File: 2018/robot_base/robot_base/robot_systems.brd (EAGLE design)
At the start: 102.8 x 91.4 mm, 92 parts, among them IC1 DRV8840PWP, IC1_C1 0.01uF, IC1_C2 0.1uF, IC1_C3 0.1uF, IC1_C4 0.1uF, IC1_C5 100uF, IC1_C6 470nF, IC1_R1 ???, IC1_R2 ???, IC1_R3 10k, IC1_R4 100m, IC1_R5 1M, IC2 DRV8840PWP, IC2_C1 0.01uF, IC2_C2 0.1uF, IC2_C3 0.1uF, IC2_C4 0.1uF, IC2_C5 100uF, IC2_C6 470nF, IC2_R1 ???, IC2_R2 ???, IC2_R3 10k, IC2_R4 100m, IC2_R5 1M, IC3 DRV8840PWP, IC3_C1 0.01uF, IC3_C2 0.1uF, IC3_C3 0.1uF, IC3_C4 0.1uF, IC3_C5 100uF, IC3_C6 470nF, IC3_R1 ???, IC3_R2 ???, IC3_R3 10k, IC3_R4 100m, IC3_R5 1M

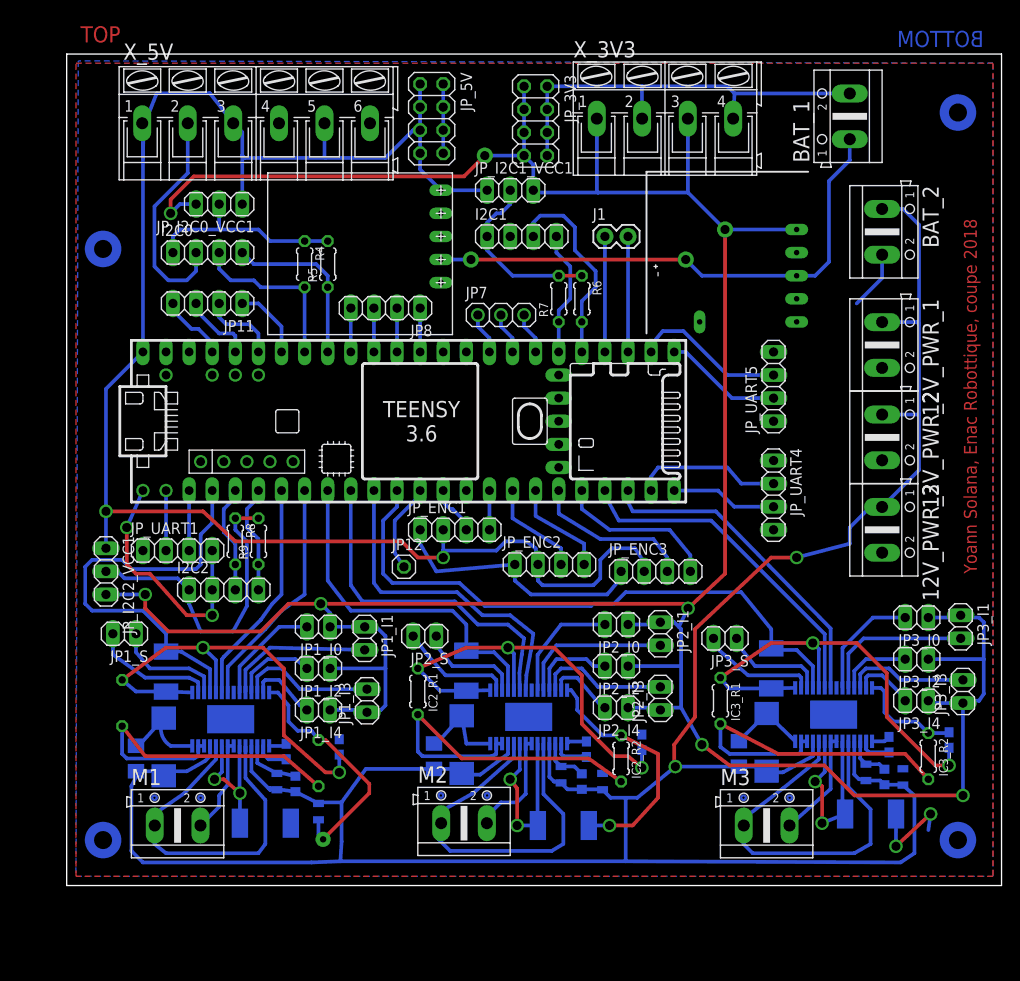
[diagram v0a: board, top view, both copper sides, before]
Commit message: Debut test motor control
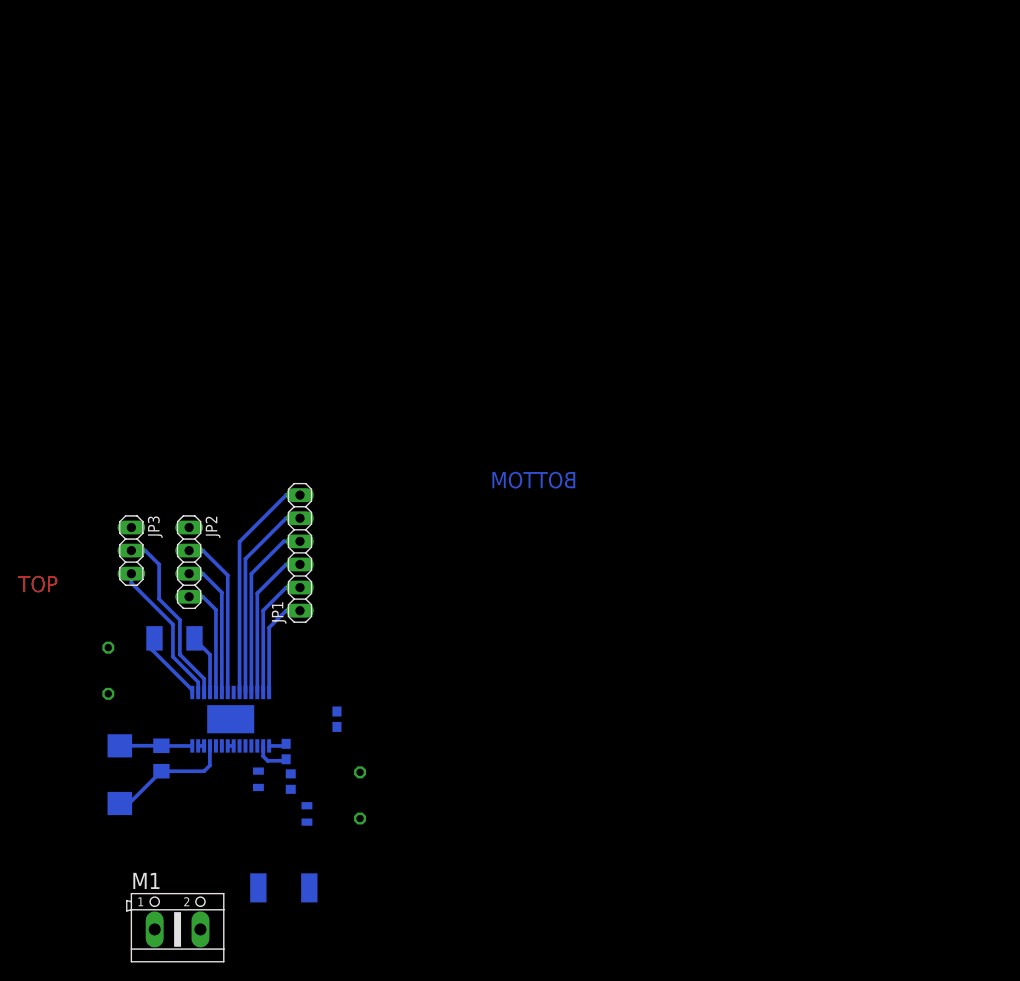
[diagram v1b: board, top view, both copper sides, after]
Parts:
- removed 12V_PWR_1, 12V_PWR_2, 12V_PWR_3, BAT_1, BAT_2, M2, M3: (no value), con-ptr500:AK500/2
- removed D24V22F3: D24V22F3, D24V22F3:D24V22F3
- removed D24V50F5: D24V50F5, D24V50F5:D24V50F5
- removed I2C0, I2C1, I2C2, JP11, JP8, JP_ENC1, JP_ENC2, JP_ENC3, JP_UART1, JP_UART4, JP_UART5: (no value), pinhead:1X04
- removed IC2, IC3: DRV8840PWP, DRV8840PWP:SOP65P640X120-29N
- removed IC2_C1, IC3_C1: 0.01uF, rcl:C0603
- removed IC2_C2, IC2_C3, IC3_C2, IC3_C3: 0.1uF, SparkFun-Passives:0805
- removed IC2_C4, IC3_C4: 0.1uF, SparkFun-Passives:1206
- removed IC2_C5, IC3_C5: 100uF, SparkFun-Passives:EIA7343
- removed IC2_C6, IC3_C6: 470nF, rcl:C0603
- removed IC2_R1, IC2_R2, IC3_R1, IC3_R2: ???, resistor:0204/5
- removed IC2_R3, IC3_R3: 10k, rcl:R2010
- removed IC2_R4, IC3_R4: 100m, rcl:R2512
- removed IC2_R5, IC3_R5: 1M, rcl:R0603
- removed J1: (no value), SparkFun-Connectors:1X02
- removed JP12: (no value), pinhead:1X01
- removed JP1_I0, JP1_I1, JP1_I2, JP1_I3, JP1_I4, JP1_S, JP2_I0, JP2_I1, JP2_I2, JP2_I3, JP2_I4, JP2_S, JP3_I0, JP3_I1, JP3_I2, JP3_I3, JP3_I4, JP3_S: (no value), pinhead:1X02
- removed JP7: (no value), adafruit:1X03
- removed JP_3V3, JP_5V: (no value), pinhead:2X04
- removed JP_I2C0_VCC1, JP_I2C1_VCC1, JP_I2C2_VCC1: (no value), pinhead:1X03
- removed R4, R5, R6, R7, R8, R9: (no value), rcl:0204/5
- removed U$1: TEENSY_3.5/3.6TEENSY_3.5/3.6_LONG_PADS, Teensy356:TEENSY_3.5/3.6
- removed X_3V3: (no value), con-ptr500:AK300/4
- removed X_5V: (no value), con-ptr500:AK300/6
- added JP1: (no value), pinhead:1X06
- added JP2: (no value), pinhead:1X04
- added JP3: (no value), pinhead:1X03
- moved M1 11.4 mm to (12.2, -4.83)
- moved IC1_R4 7.40 mm to (23.9, -0.25)
- moved IC1_R2 5.79 mm to (32.3, 9.91)
- moved IC1_C5 5.71 mm to (5.84, 12.2)
- moved IC1_R1 3.87 mm to (4.57, 23.6)
- moved IC1_R3 3.76 mm to (11.8, 27.2), turned to 0 degrees
- moved IC1_C6 3.06 mm to (29.7, 18.3)
- moved IC1_C4 2.79 mm to (10.4, 14.0)
- moved IC1_C2 2.05 mm to (21.1, 11.7)
- moved IC1_C3 1.30 mm to (26.4, 7.87)
- moved IC1_R5 0.57 mm to (24.6, 11.4)
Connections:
- removed net 3V3: D24V22F3.VOUT, JP1_I0.1, JP1_I1.1, JP1_I2.1, JP1_I3.1, JP1_I4.1, JP2_I0.1, JP2_I1.1, JP2_I2.1, JP2_I3.1, JP2_I4.1, JP3_I0.1, JP3_I1.1, JP3_I2.1, JP3_I3.1, JP3_I4.1, JP_3V3.1, JP_3V3.3, JP_3V3.5, JP_3V3.7, JP_I2C0_VCC1.3, JP_I2C1_VCC1.3, JP_I2C2_VCC1.3, X_3V3.1, X_3V3.3
- removed net 5V: D24V50F5.VOUT, JP_5V.1, JP_5V.3, JP_5V.5, JP_5V.7, JP_ENC1.2, JP_ENC2.2, JP_ENC3.2, JP_I2C0_VCC1.1, JP_I2C1_VCC1.1, JP_I2C2_VCC1.1, U$1.VIN, X_5V.1, X_5V.3, X_5V.5
- removed net CUR1_NF: JP11.1, U$1.20/A6
- removed net CUR1_SE: JP8.4, U$1.17/A3
- removed net CUR2_NF: JP8.3, U$1.16/A2
- removed net CUR2_SE: JP8.2, U$1.15/A1
- removed net CUR3_NF: JP8.1, U$1.14/A0
- removed net ENC1_A: JP_ENC1.3, U$1.12/MISO
- removed net ENC1_B: JP_ENC1.4, U$1.24
- removed net ENC2_A: JP_ENC2.3, U$1.25
- removed net ENC2_B: JP_ENC2.4, U$1.26
- removed net ENC3_A: JP_ENC3.3, U$1.27
- removed net ENC3_B: JP_ENC3.4, U$1.28
- removed net I2C0_VCC: I2C0.1, JP_I2C0_VCC1.2, R4.1, R5.2
- removed net I2C1_VCC: I2C1.1, JP_I2C1_VCC1.2, R6.1, R7.2
- removed net I2C2_VCC: I2C2.1, JP_I2C2_VCC1.2, R8.1, R9.2
- removed net IC2_I0: IC2.23, JP2_I0.2
- removed net IC2_I1: IC2.24, JP2_I1.2
- removed net IC2_I2: IC2.25, JP2_I2.2
- removed net IC2_I3: IC2.26, JP2_I3.2
- removed net IC2_I4: IC2.27, JP2_I4.2
- removed net IC2_NFAULT: IC2.18, IC2_R3.1, U$1.7
- removed net IC2_NRESET: IC2.16, JP2_S.2
- removed net IC2_NSLEEP: IC2.17, JP2_S.1
- removed net IC2_V3P3: IC2.15, IC2.19, IC2_C6.1, IC2_R1.1, IC2_R3.2
- removed net IC3_I0: IC3.23, JP3_I0.2
- removed net IC3_I1: IC3.24, JP3_I1.2
- removed net IC3_I2: IC3.25, JP3_I2.2
- removed net IC3_I3: IC3.26, JP3_I3.2
- removed net IC3_I4: IC3.27, JP3_I4.2
- removed net IC3_NFAULT: IC3.18, IC3_R3.1, U$1.10/CS
- removed net IC3_NRESET: IC3.16, JP3_S.2
- removed net IC3_NSLEEP: IC3.17, JP3_S.1
- removed net IC3_R2: IC3.12, IC3.13, IC3_R1.2, IC3_R2.2
- removed net IC3_V3P3: IC3.15, IC3.19, IC3_C6.1, IC3_R1.1, IC3_R3.2
- removed net M2_1: IC2.10, IC2.5, M2.1
- removed net M2_2: IC2.7, IC2.8, M2.2
- removed net M3_1: IC3.10, IC3.5, M3.1
- removed net M3_2: IC3.7, IC3.8, M3.2
- removed net MOT2_DIR: IC2.20, U$1.8
- removed net MOT2_PWM: IC2.21, U$1.9/CS
- removed net MOT3_DIR: IC3.20, U$1.29
- removed net MOT3_PWM: IC3.21, U$1.30
- removed net N$1: JP11.4, U$1.23/A9
- removed net N$13: IC2.1, IC2_C1.1
- removed net N$14: IC2.2, IC2_C1.2
- removed net N$15: IC2.3, IC2_C2.2, IC2_R5.2
- removed net N$17: IC3.6, IC3.9, IC3_R4.2
- removed net N$18: IC3.1, IC3_C1.1
- removed net N$19: IC3.2, IC3_C1.2
- removed net N$20: IC3.3, IC3_C2.2, IC3_R5.2
- removed net N$3: IC2.12, IC2.13, IC2_R1.2, IC2_R2.2
- removed net N$4: JP11.3, U$1.22/A8
- removed net N$52: JP7.1, U$1.A22/DAC1
- removed net N$53: JP7.2, U$1.21/DAC0
- removed net N$57: J1.1, U$1.36/A17
- removed net N$58: J1.2, U$1.35/A16
- removed net N$6: JP11.2, U$1.21/A7
- removed net N$7: JP12.1, U$1.11/MOSI
- removed net N$8: BAT_1.1, D24V22F3.VIN, D24V50F5.VIN
- removed net N$9: IC2.6, IC2.9, IC2_R4.2
- removed net NS50: JP7.3, U$1.39/A20
- removed net RX1: JP_UART1.2, U$1.0/RX
- removed net RX4: JP_UART4.2, U$1.31/A12
- removed net RX5: JP_UART5.3, U$1.34/A15
- removed net SCL0: I2C0.3, R4.2, U$1.19/A5/SCL
- removed net SCL1: I2C1.3, R6.2, U$1.37/A18
- removed net SCL2: I2C2.3, R8.2, U$1.3/CANTX
- removed net SDA0: I2C0.4, R5.1, U$1.18/A4/SDA
- removed net SDA1: I2C1.4, R7.1, U$1.38/A19
- removed net SDA2: I2C2.4, R9.1, U$1.4/CANRX
- removed net TX1: JP_UART1.3, U$1.1/TX
- removed net TX4: JP_UART4.3, U$1.32/A13
- removed net TX5: JP_UART5.2, U$1.33/A14
- new net DECAY: IC1.19, JP2.4
- net 12V2: no longer 12V_PWR_1.1, 12V_PWR_2.1, 12V_PWR_3.1, BAT_2.1, IC2.11, IC2.4, IC2_C2.1, IC2_C3.2, IC2_C4.2, IC2_C5.A, IC2_R5.1, IC3.11, IC3.4, IC3_C2.1, IC3_C3.2, IC3_C4.2, IC3_C5.A, IC3_R5.1
- net GND: now also JP1.1, JP2.1, JP3.1; no longer 12V_PWR_1.2, 12V_PWR_2.2, 12V_PWR_3.2, BAT_1.2, BAT_2.2, D24V22F3.GND, D24V22F3.GND_2, D24V22F3.PG, D24V50F5.GND, D24V50F5.GND_2, I2C0.2, I2C1.2, I2C2.2, IC2.14, IC2.28, IC2.29, IC2_C3.1, IC2_C4.1, IC2_C5.C, IC2_C6.2, IC2_R2.1, IC2_R4.1, IC3.14, IC3.28, IC3.29, IC3_C3.1, IC3_C4.1, IC3_C5.C, IC3_C6.2, IC3_R2.1, IC3_R4.1, JP_3V3.2, JP_3V3.4, JP_3V3.6, JP_3V3.8, JP_5V.2, JP_5V.4, JP_5V.6, JP_5V.8, JP_ENC1.1, JP_ENC2.1, JP_ENC3.1, JP_UART1.4, JP_UART4.4, JP_UART5.1, U$1.AGND, U$1.GND, U$1.GND2, X_3V3.2, X_3V3.4, X_5V.2, X_5V.4, X_5V.6
- net IC1_I0: now also JP1.6; no longer JP1_I0.2
- net IC1_I1: now also JP1.5; no longer JP1_I1.2
- net IC1_I2: now also JP1.4; no longer JP1_I2.2
- net IC1_I3: now also JP1.3; no longer JP1_I3.2
- net IC1_I4: now also JP1.2; no longer JP1_I4.2
- net IC1_NFAULT: no longer U$1.2
- net IC1_NRESET: now also JP3.3; no longer JP1_S.2
- net IC1_NSLEEP: now also JP3.2; no longer JP1_S.1
- net IC1_V3P3: no longer IC1.19
- net MOT1_DIR: now also JP2.3; no longer U$1.5
- net MOT1_PWM: now also JP2.2; no longer U$1.6
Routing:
- net 3V3: track 347.7 -> 0.00 mm, vias 8 -> 0
- net 12V2: track 301.1 -> 13.8 mm, vias 2 -> 0
- net GND: track 248.5 -> 19.3 mm, vias 6 -> 0
- net 5V: track 191.1 -> 0.00 mm, vias 2 -> 0
- net IC3_NFAULT: track 66.3 -> 0.00 mm
- net N$8: track 58.5 -> 0.00 mm, vias 2 -> 0
- net IC3_V3P3: track 50.7 -> 0.00 mm, vias 2 -> 0
- net IC2_V3P3: track 49.5 -> 0.00 mm, vias 2 -> 0
- net IC1_V3P3: track 51.1 -> 7.88 mm, vias 2 -> 0
- net M2_1: track 42.4 -> 0.00 mm
- net M3_1: track 42.3 -> 0.00 mm
- net N$3: track 39.9 -> 0.00 mm
- net IC1_NFAULT: track 46.5 -> 6.77 mm
- net M1_1: track 38.6 -> 0.00 mm
- net IC3_R2: track 38.5 -> 0.00 mm
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- removed copper zone on layer 1, net GND
- removed copper zone on layer 16, net GND
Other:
- board outline removed
- board text removed: "Yoann Solana, Enac Robottique, coupe 2018"
